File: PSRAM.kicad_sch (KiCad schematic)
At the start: 5 parts, among them U901 S27KL0642DPBHB023

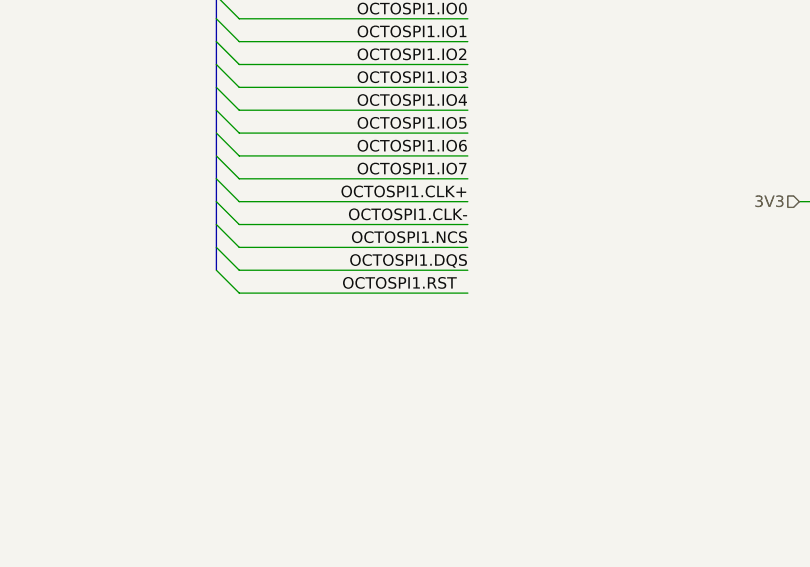
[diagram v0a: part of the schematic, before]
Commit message: more work
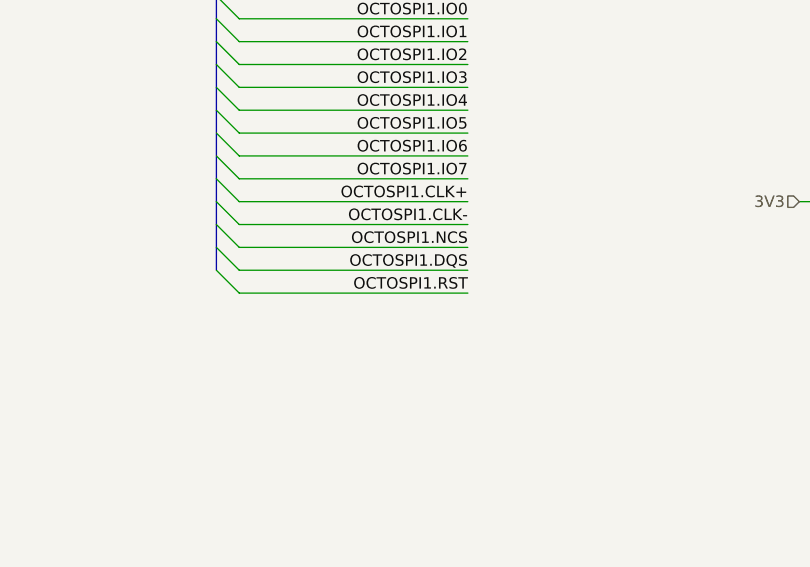
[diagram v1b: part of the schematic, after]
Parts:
- C901: JLCPCB Part Num C23692972 -> C528974
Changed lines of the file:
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@@
 	)
 	(label "OCTOSPI1.RST"
-		(at 78.74 58.42 0)
+		(at 92.71 58.42 180)
 		(effects
 			(font
 				(size 1.27 1.27)
 			)
-			(justify left bottom)
+			(justify right bottom)
 		)
 	)
@@
 			)
 		)
-		(property "JLCPCB Part Num" "C23692972"
+		(property "JLCPCB Part Num" "C528974"
 			(at 135.89 7.62 0)
 			(hide yes)
